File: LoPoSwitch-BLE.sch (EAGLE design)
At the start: 21 parts

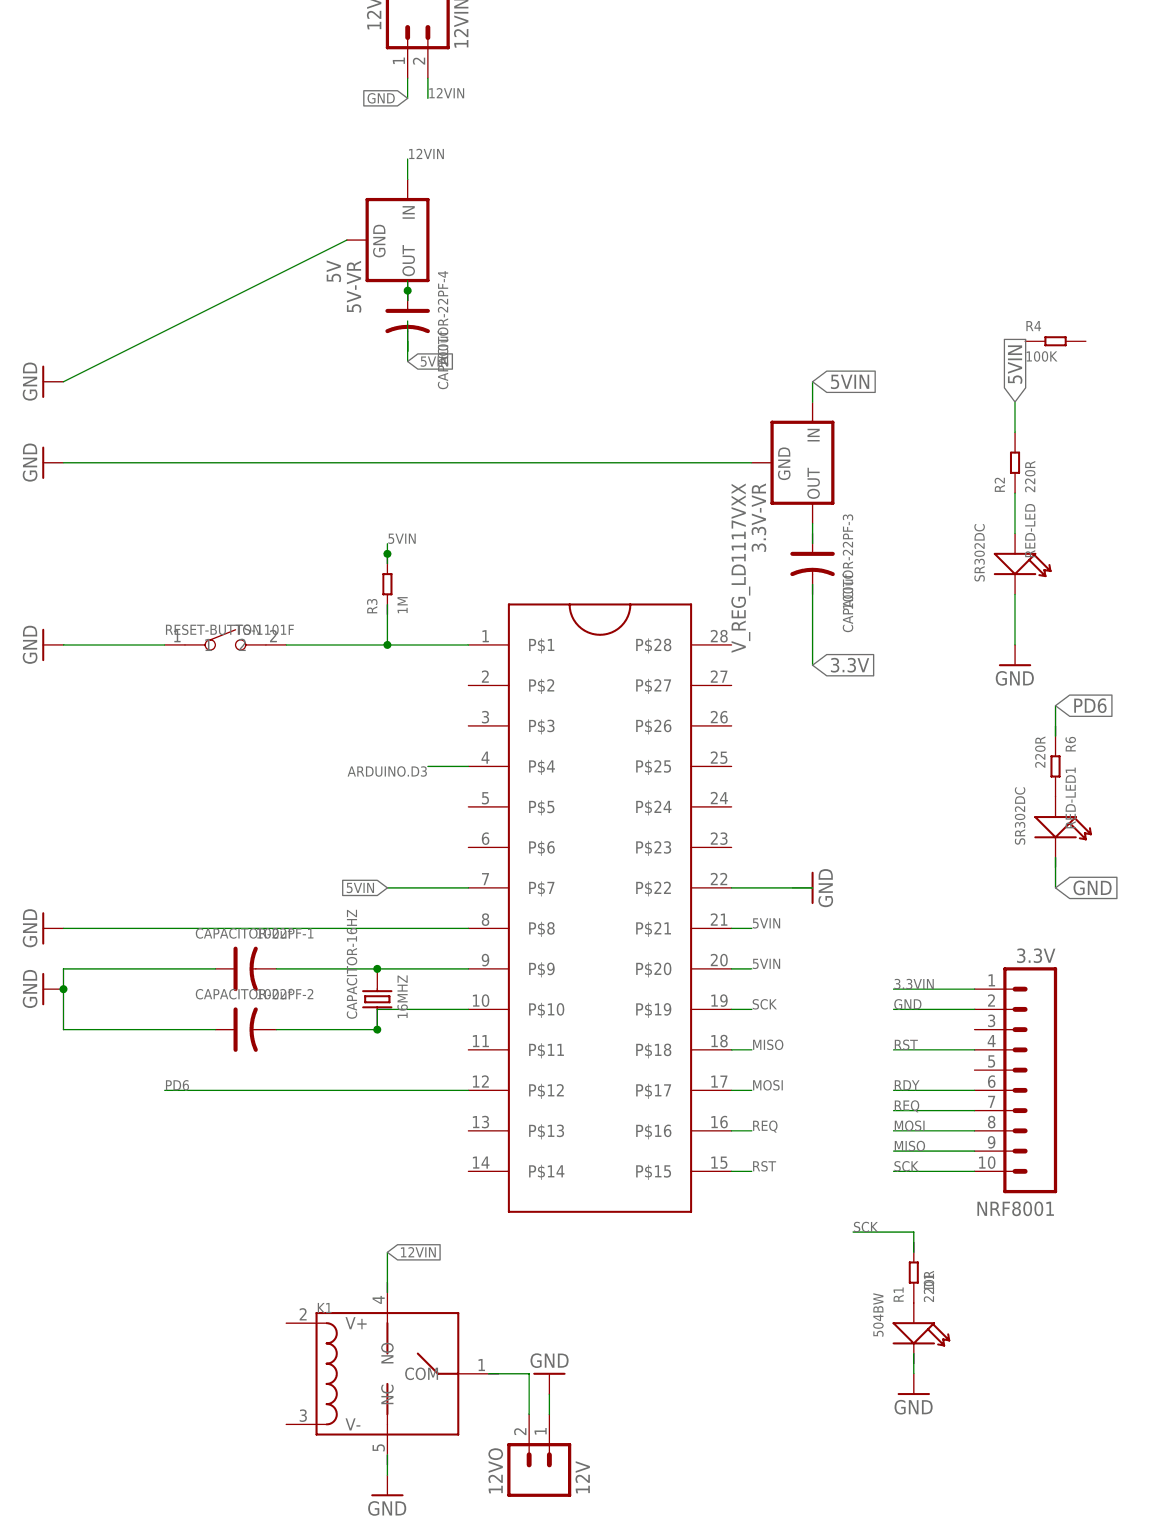
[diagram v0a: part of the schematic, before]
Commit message: Generate Seed Gerber File
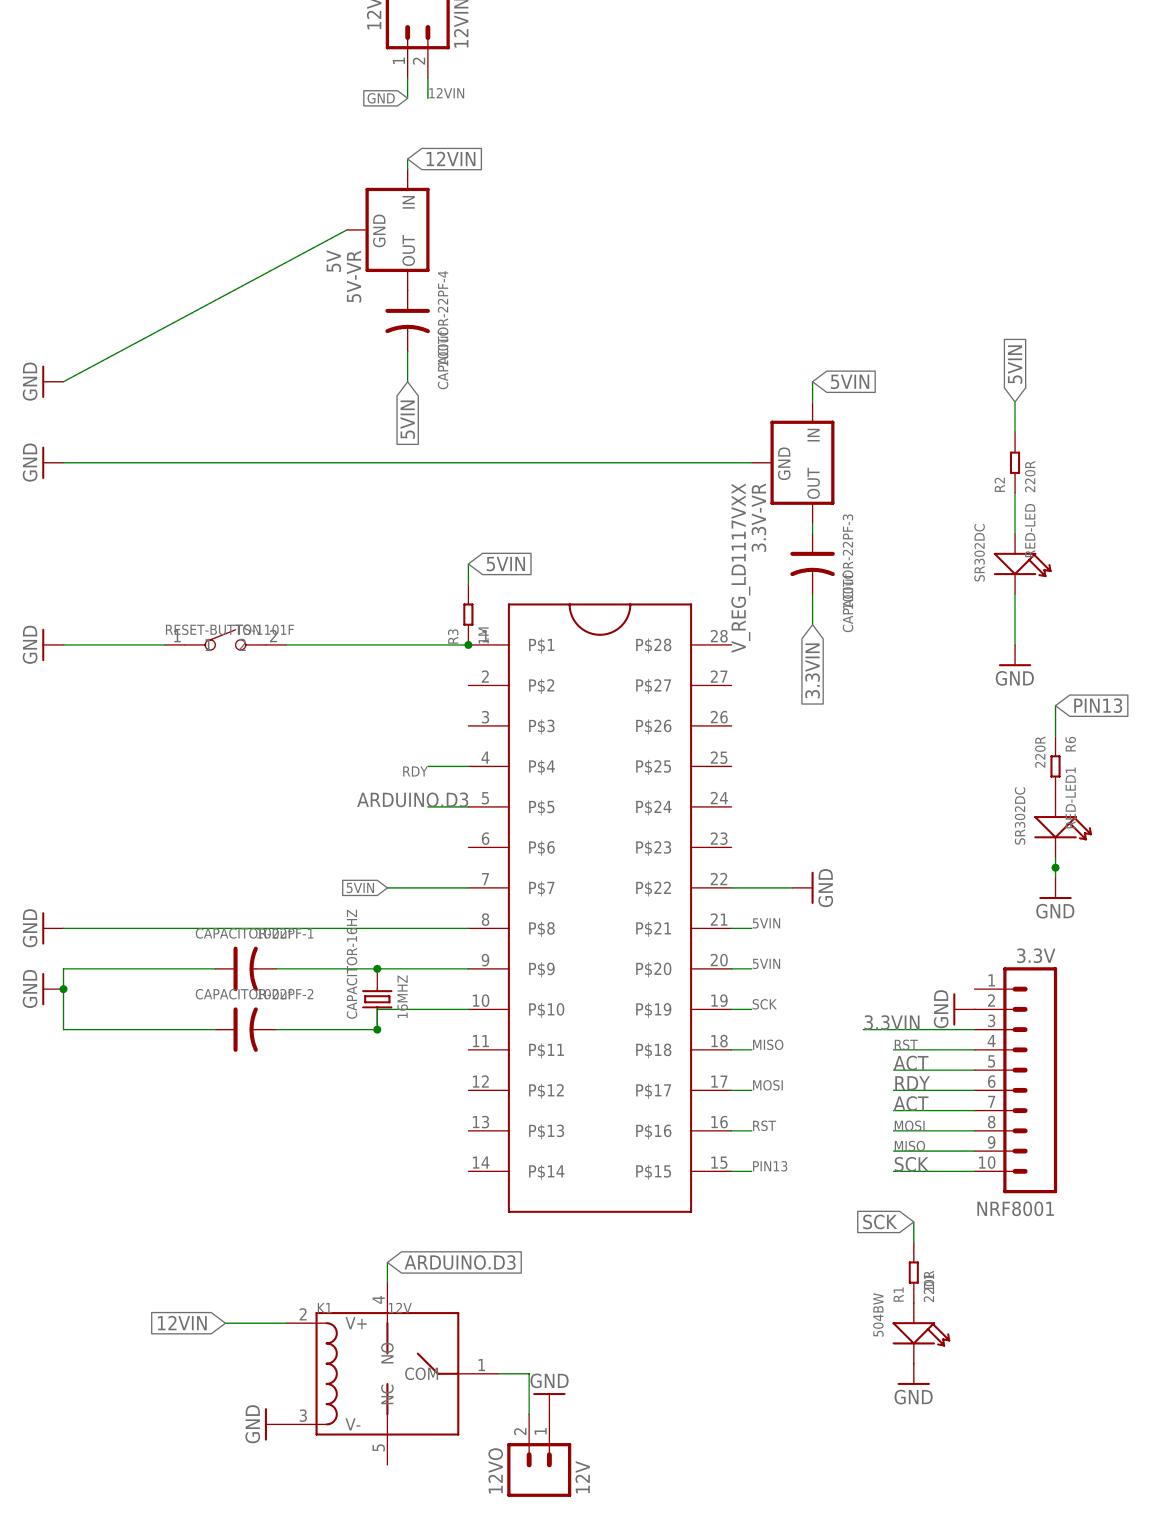
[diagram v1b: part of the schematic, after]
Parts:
- removed R4: 100K, Seeed-Resistor:DIP-RES-100K-5%-1/6W(PR-D1.8XL3.3MM)
- K1: value (none) -> 12V
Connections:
- removed net N$6: 3.3V-VR.OUT
- removed net N$9: ATMEGA328.P$22
- removed net PD6: ATMEGA328.P$12, R6.1
- removed net REQ: ATMEGA328.P$16, NRF8001.7
- new net ACT: NRF8001.5, NRF8001.7
- new net N$4: 3.3V-VR.OUT, CAPACITOR-22PF-3.+
- new net PIN13: ATMEGA328.P$15, R6.1
- net 12VIN: now also K1.V+; no longer K1.NO
- net 3.3VIN: now also CAPACITOR-22PF-3.-, NRF8001.3; no longer NRF8001.1
- net ARDUINO.D3: now also ATMEGA328.P$5, K1.NO; no longer ATMEGA328.P$4
- net GND: now also ATMEGA328.P$22, D1.-, K1.V-
- net N$1: now also K1.COM
- net N$3: now also R3.1
- net RDY: now also ATMEGA328.P$4
- net RST: now also ATMEGA328.P$16; no longer ATMEGA328.P$15
- net SCK: now also R1.2
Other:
- moved on the sheet: 5V-VR, R3

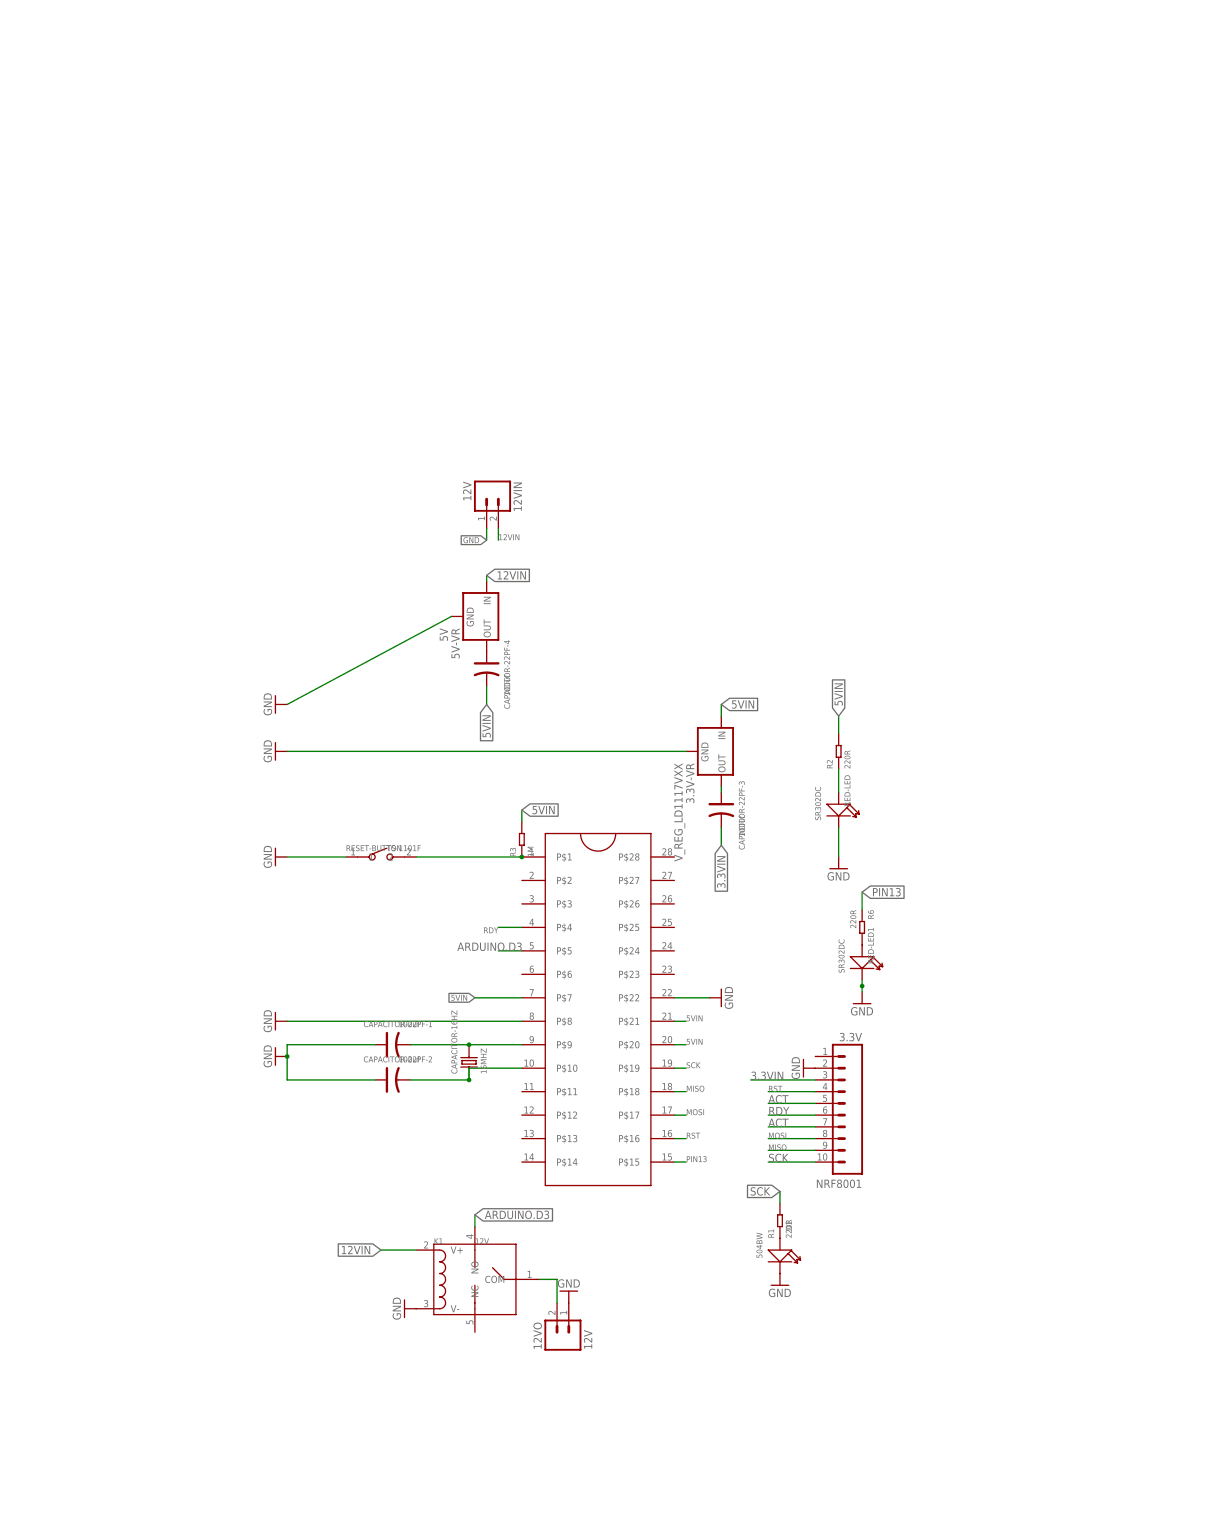
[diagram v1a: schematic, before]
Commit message: some versione
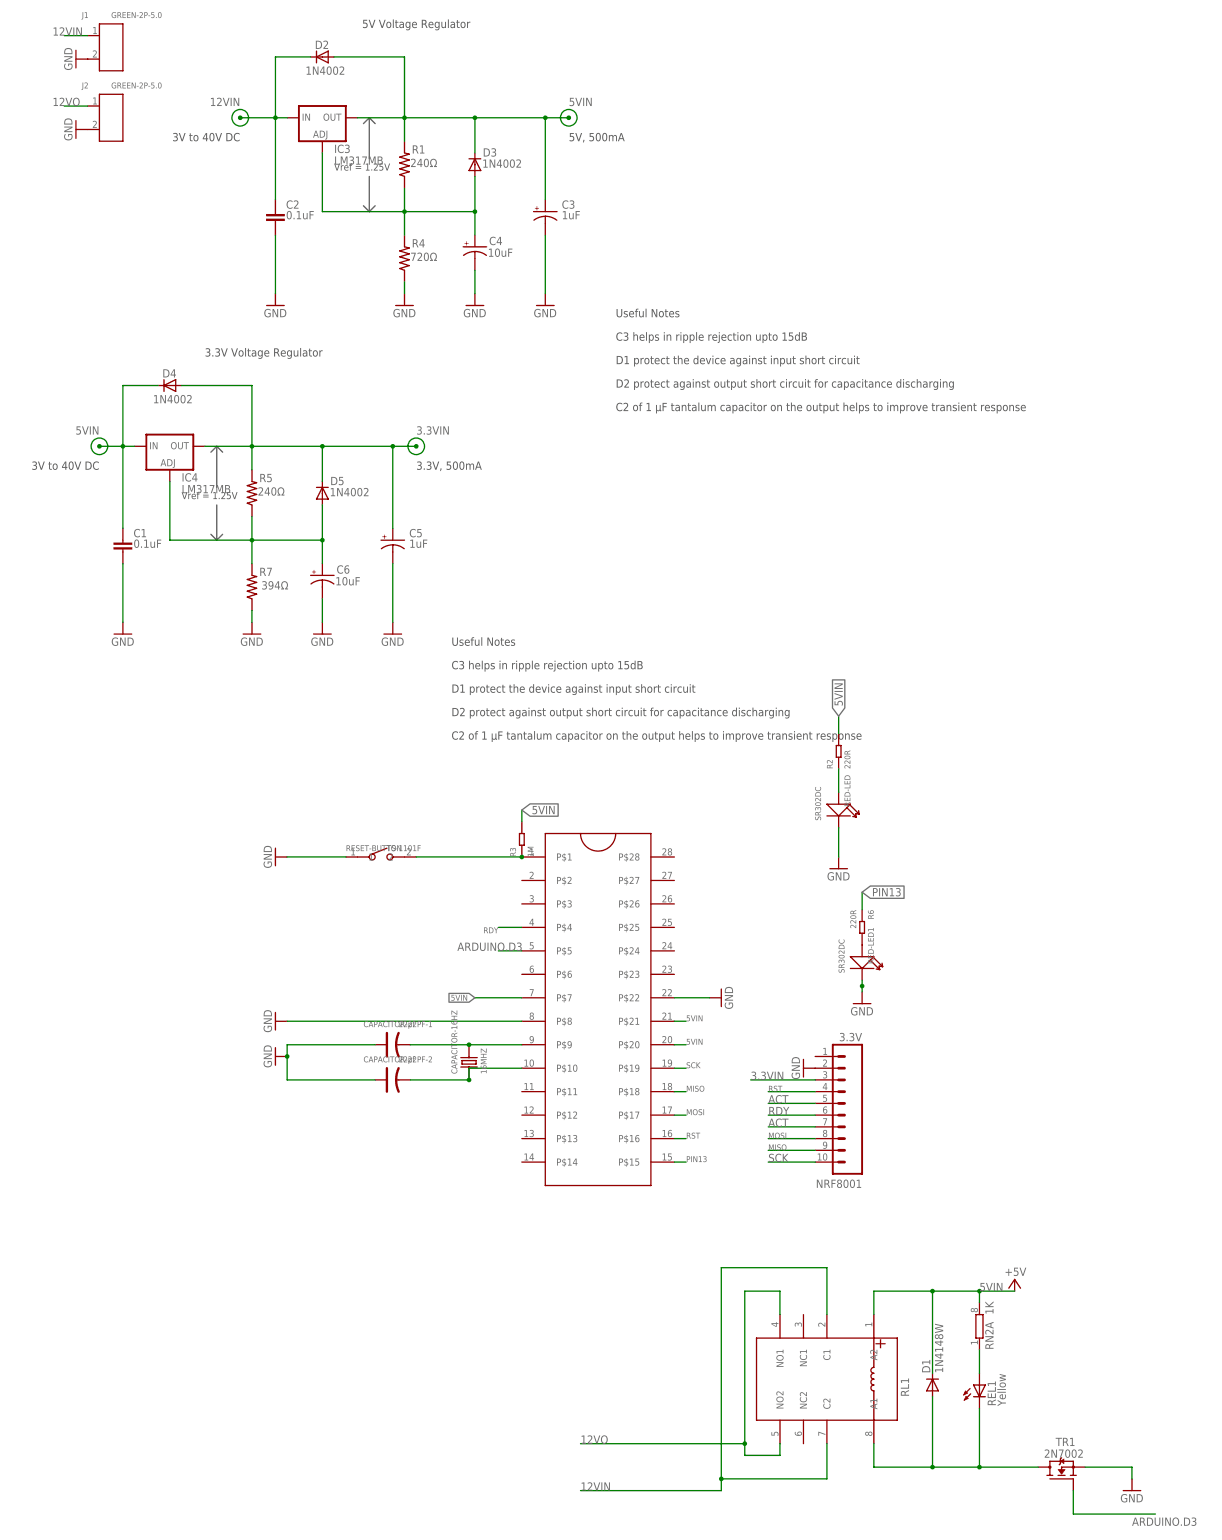
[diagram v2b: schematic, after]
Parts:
- removed 12VIN, 12VO: 12V, SparkFun-Connectors:M02JST-PTH-2
- removed 3.3V-VR: V_REG_LD1117VXX, SparkFun-PowerIC:V_REG_LD1117VXX
- removed 5V-VR: 5V, SparkFun-PowerIC:V_REG_78XX-TO-220
- removed CAPACITOR-22PF-3, CAPACITOR-22PF-4: 100uf, Seeed-Capacitor:DIP-ALUMINUM-47UF-16V(D5-H7MM)
- removed K1: 12V, Seeed-Relay:RELAY-HLS8L-DC5V-S-CHLS8L-DC5V-S-C
- added C1, C2: 0.1uF, rcl:C-EU075-052X106
- added C3, C5: 1uF, resistor:CPOL-US085CS-1AR
- added C4, C6: 10uF, resistor:CPOL-US085CS-1AR
- added D2, D3, D4, D5: 1N4002, diode:1N4004
- added IC3, IC4: LM317MB, Texas Instruments_By_element14_Batch_1:LM317MB
- added J1, J2: GREEN-2P-5.0, Seeed-Connector:SCREW-TERMINAL-GREEN(2P-5.0)
- added R4: 720Ω, resistor:R-US_M0805
- added R5: 240Ω, resistor:R-US_M0805
- added R7: 394Ω, resistor:R-US_M0805
- added REL1: Yellow, Opto:0044_KPT-2012YC
- added RL1: (no value), Rele':1045_G5V-2-H1
- added RN2: 1K, Resistenze:0005_064R_1K_/_CAY16-102J4LF
- added TR1: 2N7002, Transistors:1612_2N7002LT1G
- ATMEGA328, CAPACITOR-16HZ, NRF8001, R2, R3, R6, RED-LED, RED-LED1, RESET-BUTTON: OC_FARNELL (none) -> unknown
- CAPACITOR-22PF-1, CAPACITOR-22PF-2: value 100uf -> 22pf; OC_FARNELL (none) -> unknown
- D1: value 504BW -> 1N4148W; device Seeed-LED:DIP-LED-BLUE-BLUE(2P-D5MM) -> Diodi:0290_1N4148W; OC_FARNELL (none) -> unknown
- R1: value 220R -> 240Ω; device Seeed-Resistor:DIP-RES-220R-5%-1/4W(PR-D2.3XL6.5MM) -> resistor:R-US_M0805; OC_FARNELL (none) -> unknown
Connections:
- removed net N$7: D1.+, R1.1
- new net 12VO: J2.1, RL1.NO1, RL1.NO2
- new net N$14: D1.A, REL1.C, RL1.A1, TR1.D
- net 12VIN: now also C2.1, D2.C, IC3.IN, J1.1, RL1.C1, RL1.C2; no longer 12VIN.2, 5V-VR.IN, K1.V+
- net 3.3VIN: now also C5.+, D4.A, D5.C, IC4.OUT, R5.2; no longer CAPACITOR-22PF-3.-
- net 5VIN: now also C1.1, C3.+, D1.C, D2.A, D3.C, D4.C, IC3.OUT, IC4.IN, R1.2, RL1.A2, RN2A.2; no longer 3.3V-VR.IN, CAPACITOR-22PF-4.-
- net ARDUINO.D3: now also TR1.G; no longer K1.NO
- net GND: now also C1.2, C2.2, C3.-, C4.-, C5.-, C6.-, J1.2, J2.2, R4.1, R7.1, TR1.S; no longer 12VIN.1, 12VO.1, 3.3V-VR.GND, 5V-VR.GND, D1.-, K1.V-
- net N$1: now also C4.+, D3.A, IC3.ADJ, R1.1, R4.2; no longer 12VO.2, K1.COM
- net N$4: now also C6.+, D5.A, IC4.ADJ, R5.1, R7.2; no longer 3.3V-VR.OUT, CAPACITOR-22PF-3.+
- net N$5: now also REL1.A, RN2A.1; no longer 5V-VR.OUT, CAPACITOR-22PF-4.+
- net SCK: no longer R1.2
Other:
- note added: "3.3V Voltage Regulator"
- note added: "3.3V, 500mA"
- note added: "3V to 40V DC"
- note added: "5V Voltage Regulator"
- note added: "5V, 500mA"
- note added: "C2 of 1 µF tantalum capacitor on the output helps to improve transient response"
- note added: "C3 helps in ripple rejection upto 15dB"
- note added: "D1 protect the device against input short circuit"
- note added: "D2 protect against output short circuit for capacitance discharging"
- note added: "Useful Notes"
- note added: "Vref = 1.25V"
